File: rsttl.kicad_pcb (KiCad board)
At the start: 2 copper layers, 83.2 x 32 mm, 20 parts, among them J1 DB9_Male, J2 7-20V Ext, J3 TTL Data, 5V, J4 5V Ext SW, J5 DB9_Female, U1 L7805, U2 MAX232

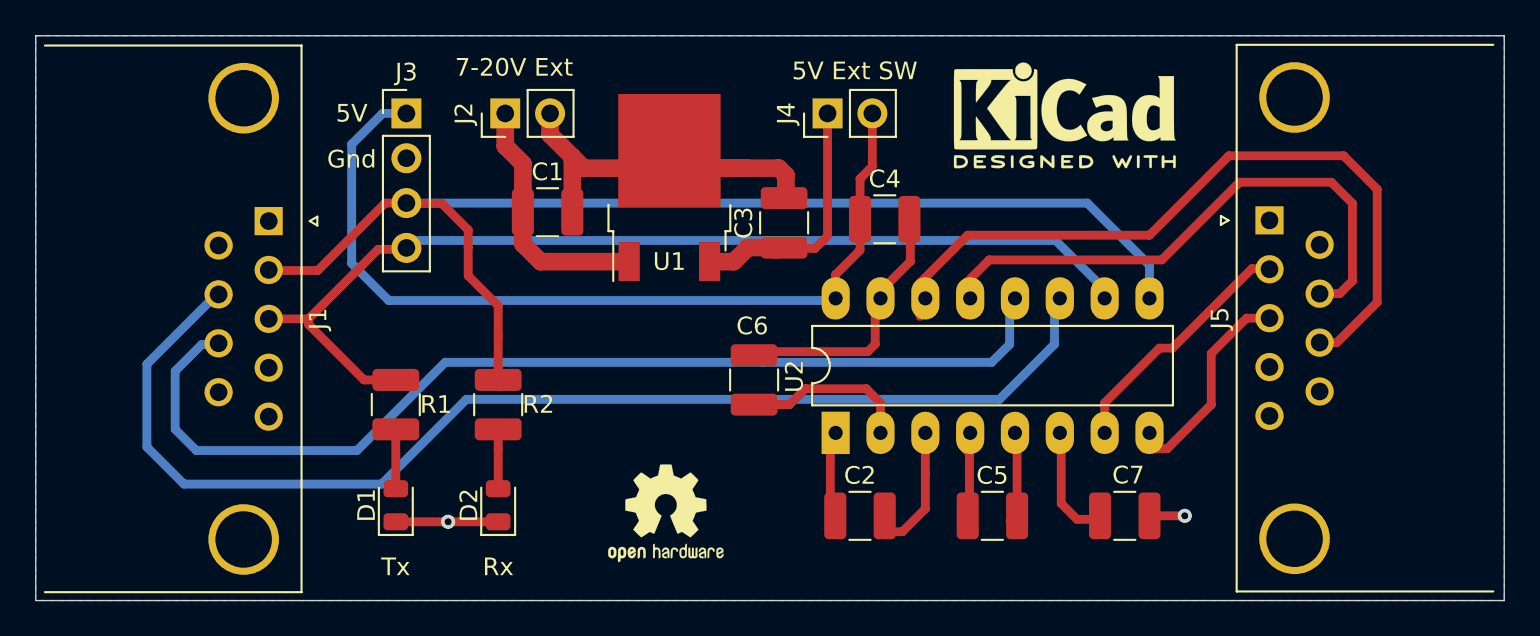
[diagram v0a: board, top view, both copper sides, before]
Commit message: Rev.B
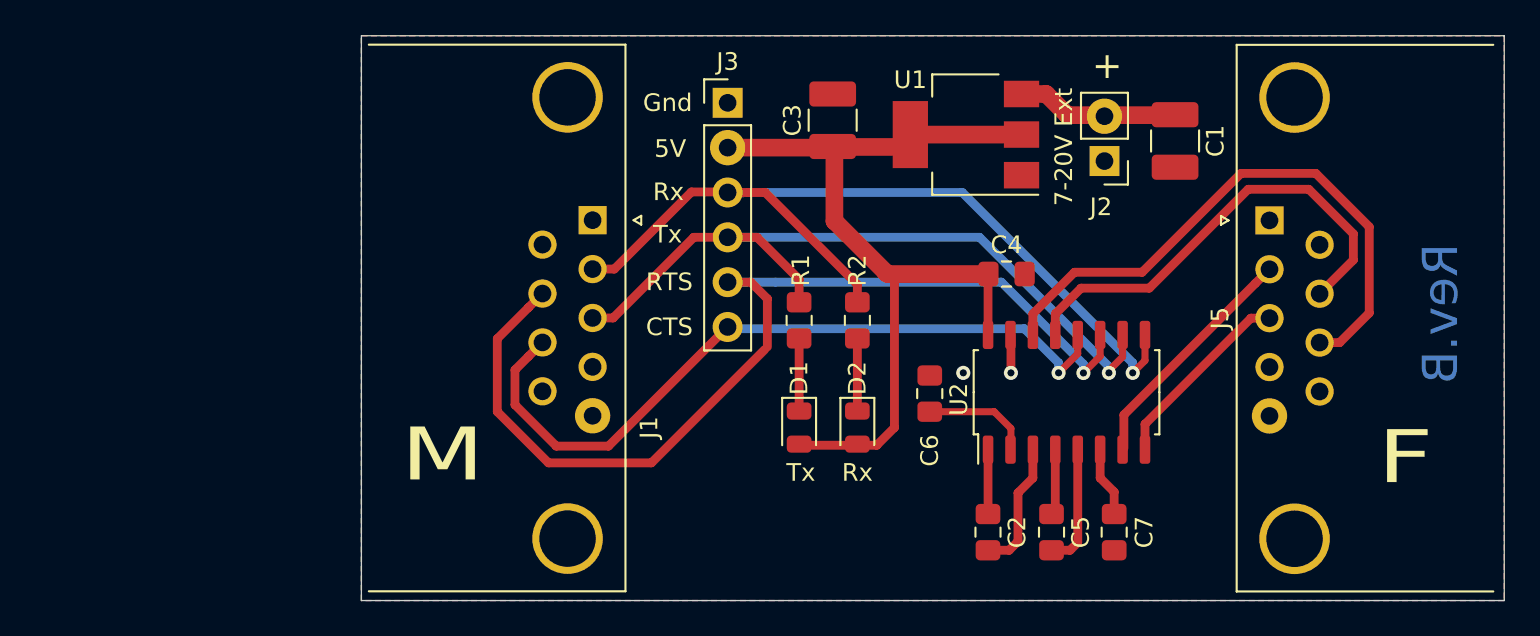
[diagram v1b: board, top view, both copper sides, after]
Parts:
- removed J4: 5V Ext SW, Connector_PinHeader_2.54mm:PinHeader_1x02_P2.54mm_Vertical
- C1, C3: footprint Capacitor_SMD:C_1210_3225Metric -> Capacitor_SMD:C_1210_3225Metric_Pad1.42x2.65mm_HandSolder
- C2, C4, C5, C6, C7: footprint Capacitor_SMD:C_1210_3225Metric -> Capacitor_SMD:C_0805_2012Metric_Pad1.15x1.40mm_HandSolder
- J3: footprint Connector_PinHeader_2.54mm:PinHeader_1x04_P2.54mm_Vertical -> Connector_PinHeader_2.54mm:PinHeader_1x06_P2.54mm_Vertical
- R1, R2: footprint Resistor_SMD:R_1210_3225Metric -> Resistor_SMD:R_0805_2012Metric_Pad1.15x1.40mm_HandSolder
- REF** (x2): moved to B.Cu
- U1: value L7805 -> NCP1117; footprint Package_TO_SOT_SMD:TO-252-2 -> Package_TO_SOT_SMD:SOT-223-3_TabPin2
- U2: footprint Package_DIP:DIP-16_W7.62mm_LongPads -> Package_SO:SOP-16_4.55x10.3mm_P1.27mm
- moved C1 35.8 mm to (149.9, 94.0), turned to 270 degrees
- moved J2 34.1 mm to (145.9, 95.1), turned to 180 degrees
- moved R1 23.3 mm to (128.7, 104.1)
- moved REF** 23.3 mm to (145.1, 115.8), turned to 180 degrees
- moved D1 23.3 mm to (128.7, 110.2), turned to 270 degrees
- moved R2 20.9 mm to (131.9, 104.1)
- moved D2 20.8 mm to (131.9, 110.2), turned to 270 degrees
- moved J1 18.4 mm to (117.0, 98.5)
- moved J3 18.2 mm to (124.6, 91.8)
- moved U1 17.1 mm to (138.1, 93.6), turned to 180 degrees
- moved U2 13.3 mm to (143.8, 108.2)
- moved C6 9.98 mm to (136.1, 108.3)
- moved C4 7.56 mm to (140.4, 101.5)
- moved C2 7.31 mm to (139.3, 116.1), turned to 270 degrees
- moved C3 6.43 mm to (130.6, 92.8)
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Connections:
- C3 pad 1: Net-(C3-Pad1) -> +5V
- D1 pad 1: GND -> Net-(D1-Pad1)
- D1 pad 2: Net-(D1-Pad2) -> +5V
- D2 pad 1: GND -> Net-(D2-Pad1)
- D2 pad 2: Net-(D2-Pad2) -> +5V
- J1 pad 1: Net-(J1-Pad1) -> (no net)
- J1 pad 4: Net-(J1-Pad4) -> (no net)
- J1 pad 6: Net-(J1-Pad6) -> (no net)
- J1 pad 9: Net-(J1-Pad9) -> (no net)
- J2 pad 1: VCC -> GND
- J2 pad 2: GND -> VCC
- J3 pad 1: +5V -> GND
- J3 pad 2: GND -> +5V
- J5 pad 1: Net-(J5-Pad1) -> (no net)
- J5 pad 4: Net-(J5-Pad4) -> (no net)
- J5 pad 6: Net-(J5-Pad6) -> (no net)
- J5 pad 9: Net-(J5-Pad9) -> (no net)
- R1 pad 2: Net-(D1-Pad2) -> Net-(D1-Pad1)
- R2 pad 2: Net-(D2-Pad2) -> Net-(D2-Pad1)
- U1 pad 1: VCC -> GND
- U1 pad 2: GND -> +5V
- U1 pad 3: Net-(C3-Pad1) -> VCC
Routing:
- net GND: track 47.5 -> 2.06 mm
- net Net-(J1-Pad2): track 70.7 -> 50.9 mm, vias 0 -> 1
- net Net-(J1-Pad8): track 58.2 -> 42.8 mm, vias 0 -> 1
- net Net-(J1-Pad3): track 57.7 -> 43.3 mm, vias 0 -> 1
- net Net-(C3-Pad1): track 13.9 -> 0.00 mm
- net Net-(J1-Pad7): track 67.6 -> 57.5 mm, vias 0 -> 1
- net Net-(J5-Pad8): track 42.2 -> 33.2 mm
- net Net-(J5-Pad7): track 33.1 -> 26.2 mm
- net VCC: track 13.5 -> 9.21 mm
- net Net-(D2-Pad1): track 0.00 -> 4.11 mm
- net Net-(D1-Pad1): track 0.00 -> 4.11 mm
- net Net-(C6-Pad1): track 10.6 -> 6.55 mm
- net Net-(D2-Pad2): track 2.80 -> 0.00 mm
- net Net-(D1-Pad2): track 2.80 -> 0.00 mm
- net Net-(C7-Pad2): track 6.51 -> 3.98 mm
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- added copper zone on F.Cu, net GND
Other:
- board size 83.2 x 32 mm -> 64.8 x 32 mm
- rule trace_min: 0.2 -> 0.4
- board text added: "+"
- board text added: "CTS"
- board text added: "F"
- board text added: "M"
- board text added: "RTS"
- board text added: "Rev.B"
- board text removed: "rev.A"
